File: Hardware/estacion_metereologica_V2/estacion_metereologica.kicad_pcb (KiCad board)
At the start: 2 copper layers, 66 x 69 mm, 24 parts, among them J1 Screw_Terminal_01x02, J2 Step_Down_Mini, J3 Conn_01x03_Pin, U1 AMS1117

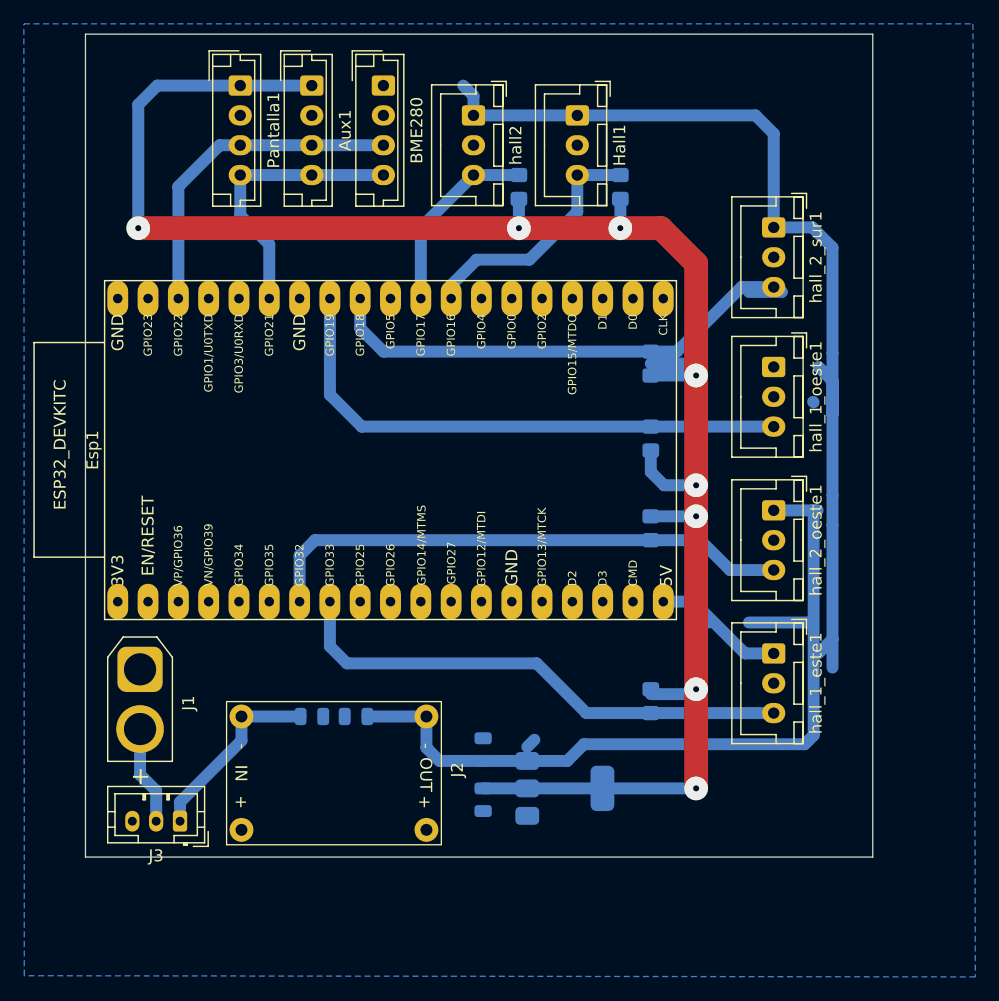
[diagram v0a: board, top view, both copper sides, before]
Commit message: Se actualizo detalles del PCB
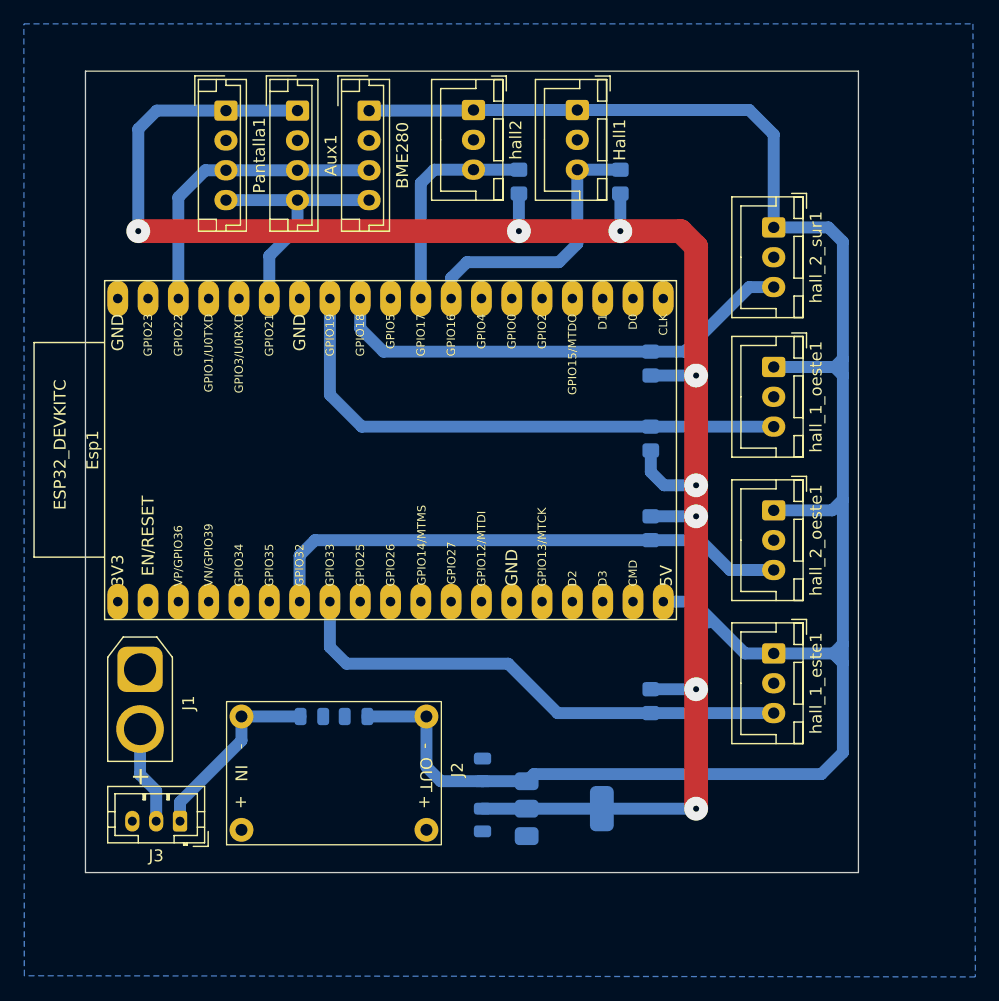
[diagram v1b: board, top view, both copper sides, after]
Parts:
- moved BME280 2.42 mm to (48.8, 25.1)
- moved Pantalla1 2.42 mm to (36.8, 25.1)
- moved Aux1 2.42 mm to (42.8, 25.1)
- moved C_0.33µF4 1.70 mm to (58.3, 84.5)
- moved C_0.33µF3 1.70 mm to (58.3, 80.3)
- moved U1 1.70 mm to (65.2, 83.6)
- moved Hall1 0.45 mm to (66.2, 25.1)
- moved R5 0.45 mm to (69.8, 31.1)
- moved R6 0.45 mm to (61.4, 31.1)
- moved hall2 0.45 mm to (57.5, 25.1)
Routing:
- net 3V3: track 186.5 -> 159.5 mm
- net SCL: track 28.0 -> 25.4 mm
- net OUT_6: track 16.0 -> 18.4 mm
- net OUT_5: track 20.9 -> 23.3 mm
- net SDA: track 23.4 -> 21.2 mm
- net VO+: track 169.9 -> 171.1 mm
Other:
- board size 66 x 69 mm -> 64.8 x 67.2 mm
